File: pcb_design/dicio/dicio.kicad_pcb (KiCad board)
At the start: 2 copper layers, 93 x 93 mm, 76 parts, among them J1 Conn_02x03_Counter_Clockwise, J2 Conn_01x06_Female, J3 USB_C_Receptacle, J4 Micro_SD_Card, J5 USB_C_Receptacle, J6 USB_C_Receptacle, J7 Conn_02x13_Odd_Even, J8 USB_C_Receptacle, Q1 Q_NMOS_GSD, SW1 SW_SPST, SW2 SW_SPST, U1 dsPIC33EP256MU806, U2 MCP2542FD, U3 S70FL01GS, U4 TPS737, U5 SiP32431, U6 SiP32431, U7 ADM7170, Y1 Crystal_GND24, Y2 Crystal_GND24

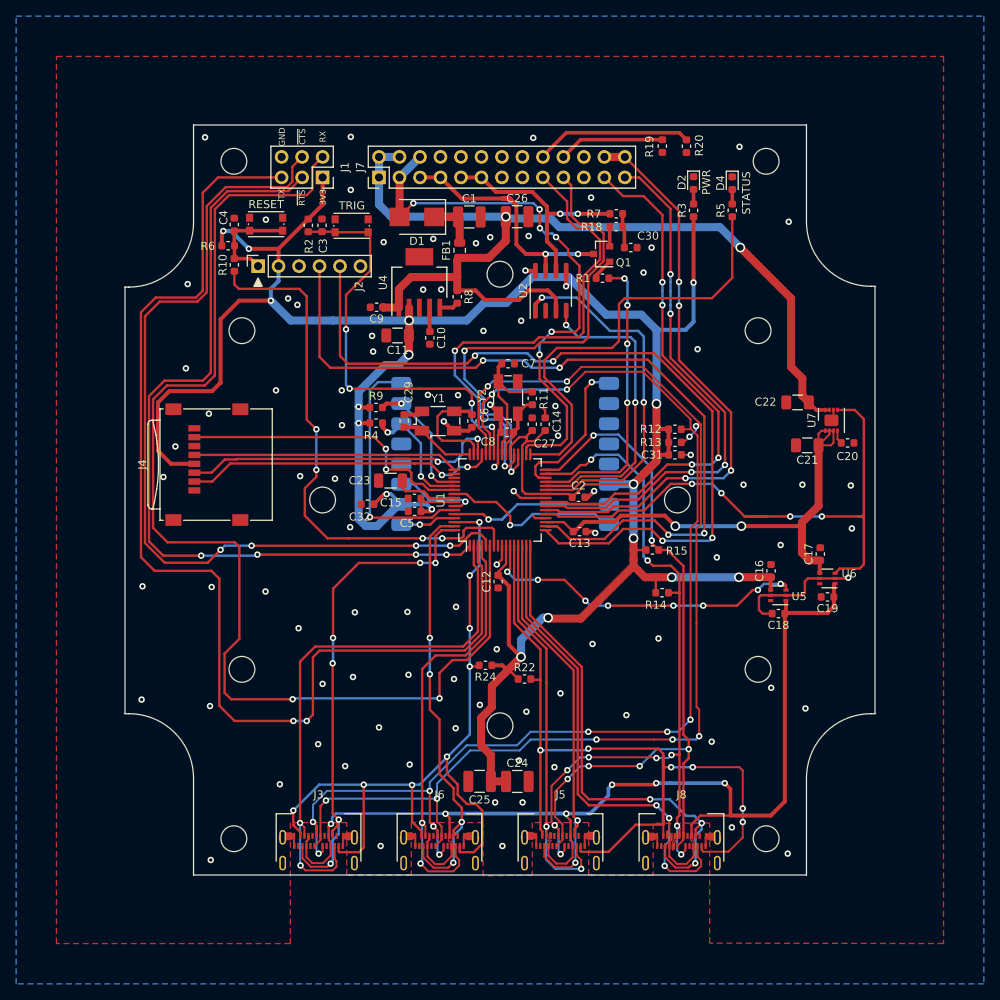
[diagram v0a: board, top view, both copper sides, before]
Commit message: Improved design.
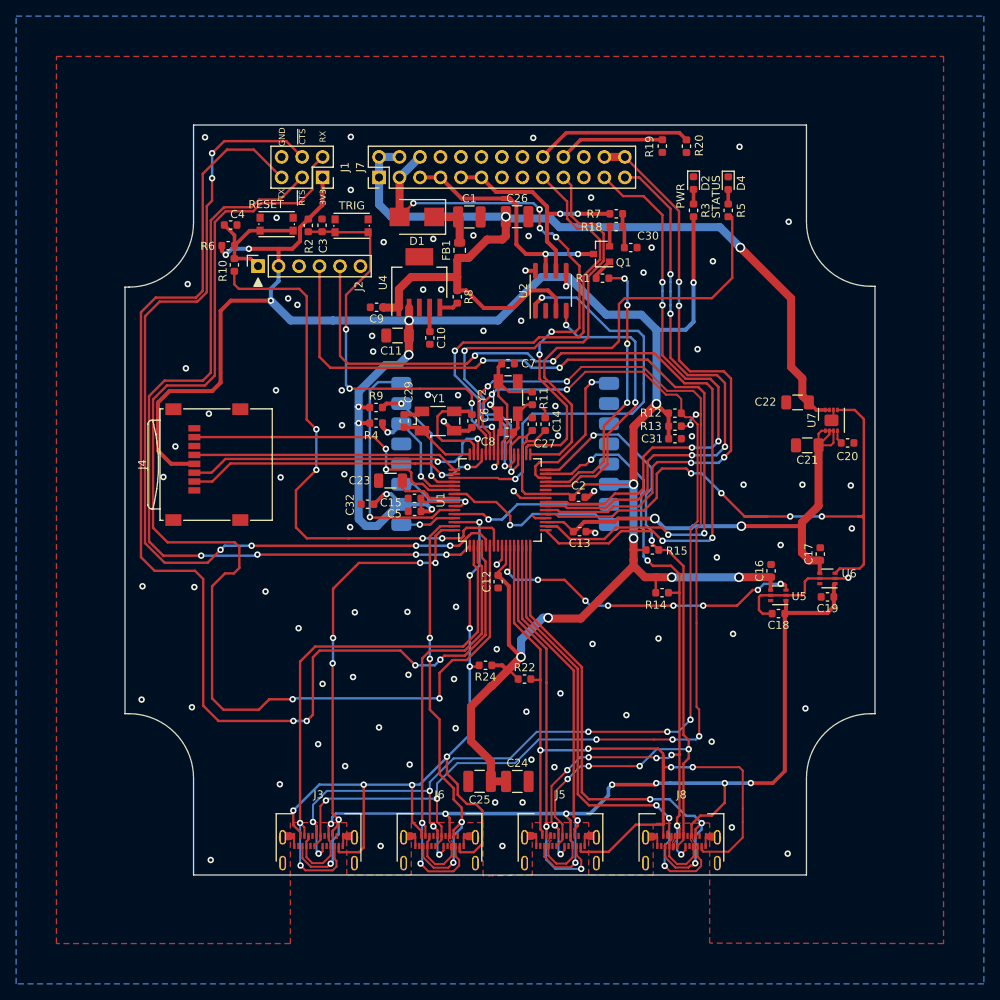
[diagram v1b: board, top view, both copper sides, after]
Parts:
- moved C31 2.00 mm to (106.7, 77.4)
- moved R12 2.00 mm to (106.7, 74.2)
- moved R13 2.00 mm to (106.7, 75.8)
- moved SW2 1.30 mm to (57.3, 50.8)
- moved D4 0.50 mm to (113.3, 45.7)
- moved R5 0.50 mm to (113.3, 49.1)
- moved C4 0.45 mm to (51.6, 50.9), turned to 0 degrees
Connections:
- U1 pad 27: /C1TX -> unconnected-(U1-Pad27)
- U1 pad 3: /U1TX -> /OW3
- U1 pad 4: /OW3 -> /U1TX
- U1 pad 51: unconnected-(U1-Pad51) -> /C1TX
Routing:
- net /C1TX: track 45.6 -> 55.7 mm
- net /U1TX: track 141.5 -> 147.8 mm, vias 2 -> 4
- net /S_PS: track 144.3 -> 139.2 mm, vias 6 -> 7
- net /~{U1CTS}: track 110.4 -> 114.4 mm, vias 4 -> 6
- net /U1RX: track 143.2 -> 146.6 mm
- net /EN_VA: track 72.4 -> 75.7 mm
- net /~{MCLR}: track 12.8 -> 16.1 mm
- net /SYNC: track 72.1 -> 75.0 mm
- net /CAN_C2: track 66.4 -> 69.3 mm
- net /CAN_C1: track 66.0 -> 68.9 mm
- net /~{MCLR_w}: track 67.1 -> 69.5 mm
- net /TERM: track 36.2 -> 34.3 mm
- net /C1RX: track 38.5 -> 36.6 mm
- net /PGC: track 100.6 -> 102.0 mm
- net GND: track 67.8 -> 66.6 mm, vias 93 -> 92
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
